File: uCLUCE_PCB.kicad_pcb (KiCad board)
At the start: 2 copper layers, 17.1 x 27.5 mm, 19 parts, among them J1 Screw_Terminal_01x03, J2 GS2, P1 USB_A, P2 UART_TTL, U1 PIC16F1455-I/ST, U2 MCP2003B-E/SN, U3 fiducial

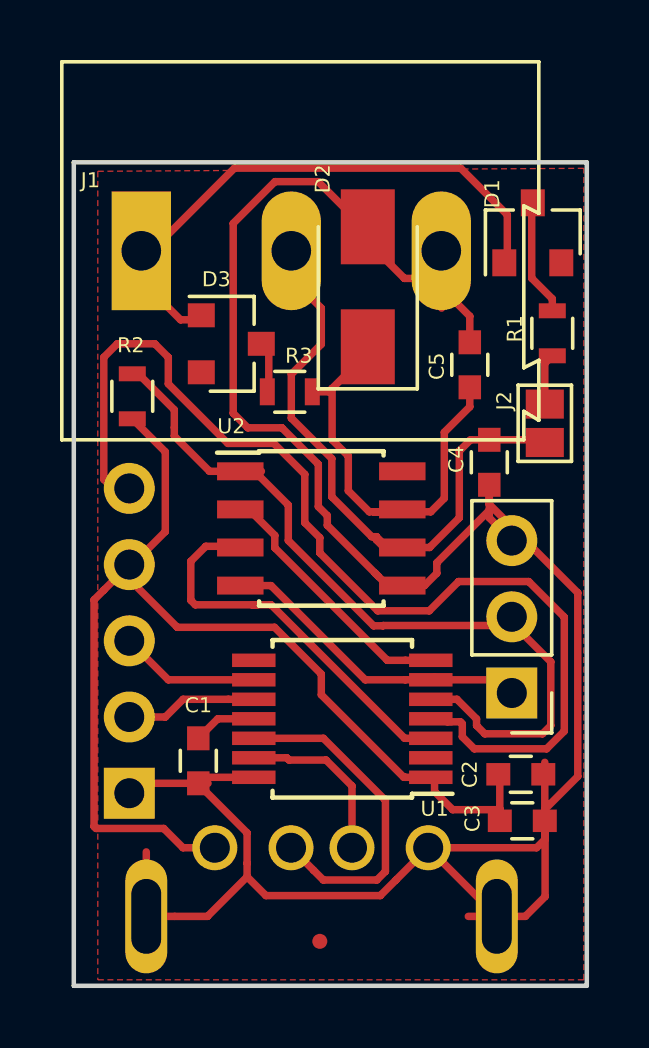
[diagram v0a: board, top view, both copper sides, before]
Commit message: Analog sw
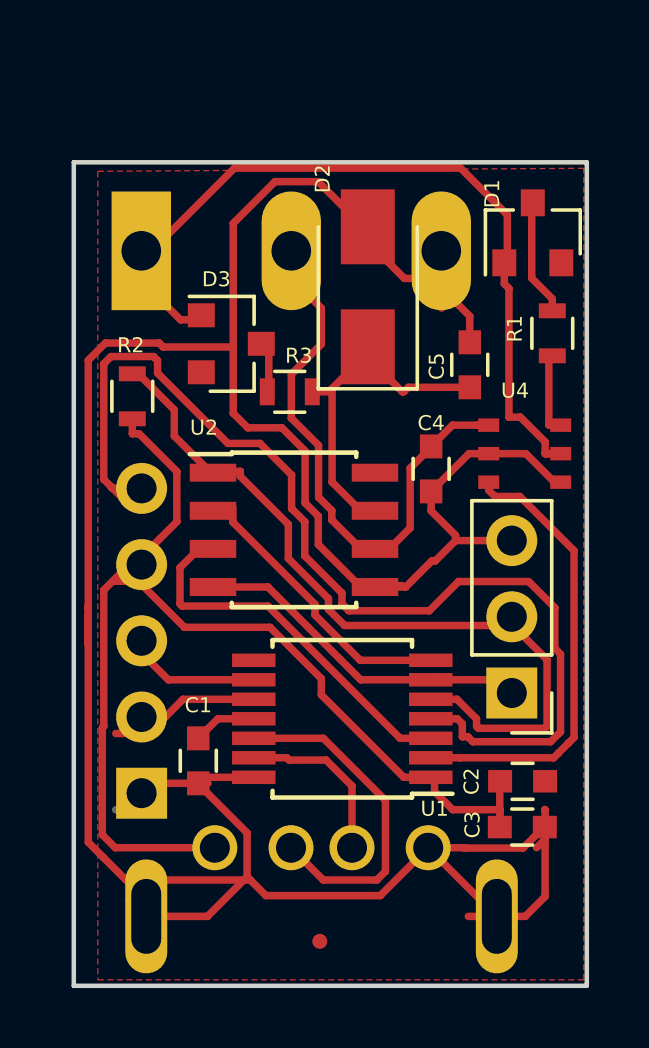
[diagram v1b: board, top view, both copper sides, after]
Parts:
- removed J2: GS2, Connectors:GS2
- added U4: DG468, uCLUCE_PCB:TSOP6, F.Cu at (53.5, 35.4)
- J1: moved to B.Cu
- moved C4 1.95 mm to (51.6, 36.8)
- moved U2 0.91 mm to (47.0, 38.9)
- moved ICS1 0.41 mm to (41.9, 47.6)
- moved C2 0.24 mm to (54.6, 47.2)
- moved C3 0.21 mm to (54.6, 48.8)
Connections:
- U1 pad 2: (no net) -> Net-(U1-Pad2)
- U1 pad 8: (no net) -> Net-(U1-Pad8)
- U2 pad 8: (no net) -> Net-(U2-Pad8)
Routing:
- net GND: track 88.0 -> 106.0 mm
- net Net-(U1-Pad2): track 0.00 -> 15.2 mm
- net +BATT: track 19.4 -> 27.2 mm
- net Net-(C5-Pad1): track 15.0 -> 12.4 mm
- net Net-(C4-Pad1): track 20.6 -> 18.0 mm
- net Net-(R1-Pad2): track 1.71 -> 2.75 mm
- net Net-(P2-Pad1): track 10.7 -> 11.6 mm
- net Net-(P2-Pad2): track 27.0 -> 26.3 mm
- net Net-(ICS1-Pad3): track 5.41 -> 4.81 mm
- net +5V: track 40.4 -> 39.8 mm

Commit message: update to Kicad 6
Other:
- net class Default removed
